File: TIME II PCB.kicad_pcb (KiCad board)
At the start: 2 copper layers, 98 x 98 mm, 91 parts, among them J1 USB_C_Receptacle, J2 SD_Card, J21 Conn_01x02_Male, J3 Conn_01x02_Male, J4 Conn_01x05_Pin, J5 Conn_01x05_Pin, J6 Conn_01x05_Pin, J7 Conn_01x05_Pin, J8 Conn_01x05_Pin, Q1 VNP10N07, Q2 VNP10N07, Q3 VNP10N07, Q4 VNP10N07, Q5 VNP10N07, Q6 NMOS, Q7 PMOS, SW1 PTS647SM38SMTR2LFS, SW2 PTS647SM38SMTR2LFS, U1 ESP32-S2-SOLO, U2 ADP2303, U3 LTC4420CMSE-PBF

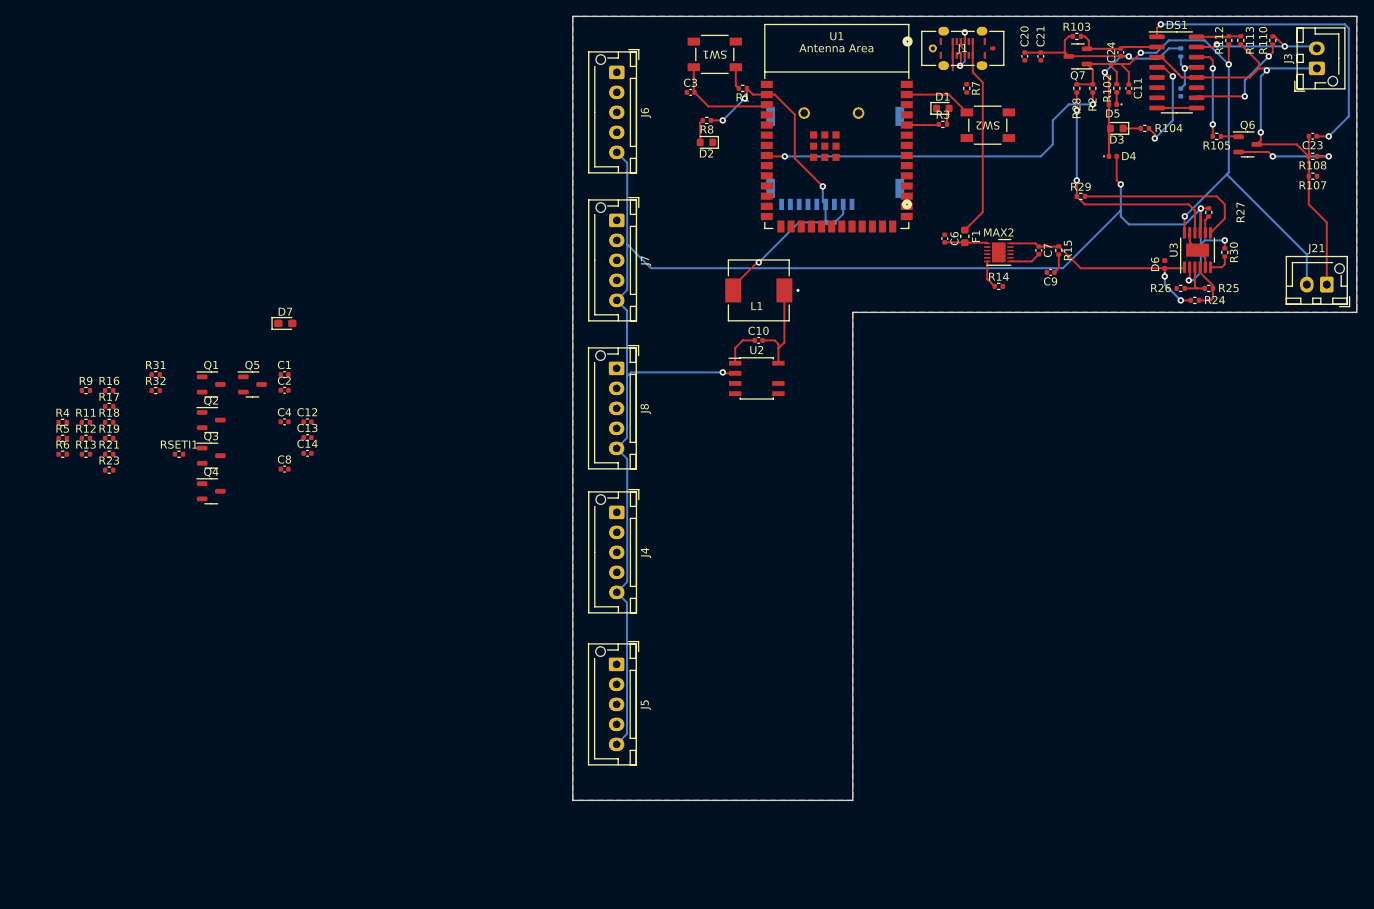
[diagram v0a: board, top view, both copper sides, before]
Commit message: motor driver
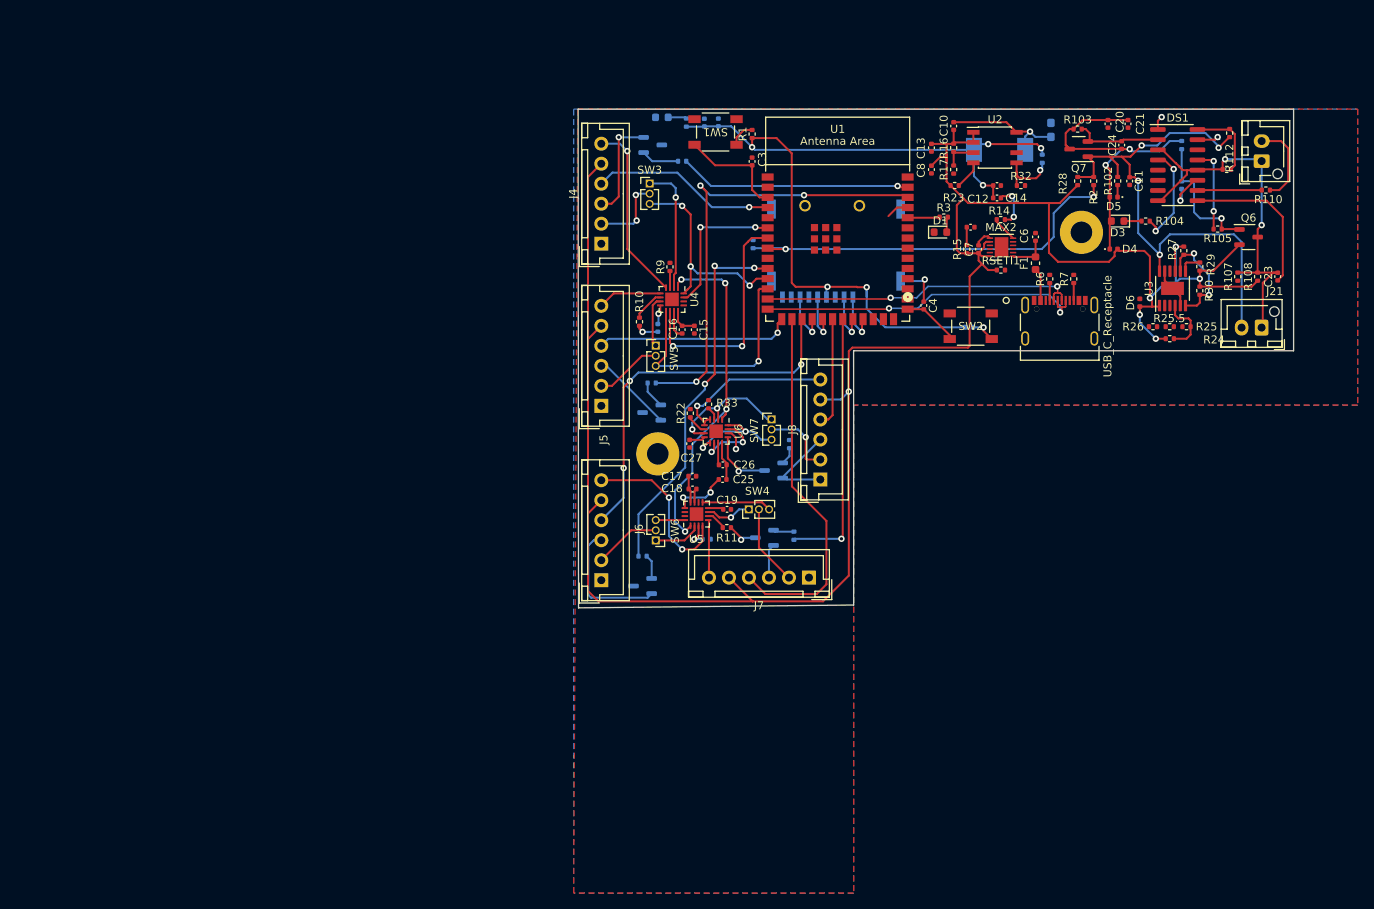
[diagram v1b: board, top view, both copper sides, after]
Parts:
- added ?: , , F.Cu at (150.6, 106.7)
- added C15: 10uF, Capacitor_SMD:C_0402_1005Metric, F.Cu at (155.2, 91.2)
- added C16: 0.01uF, Capacitor_SMD:C_0402_1005Metric, F.Cu at (153.7, 91.2)
- added C17: 10uF, Capacitor_SMD:C_0402_1005Metric, F.Cu at (154.9, 109.5)
- added C18: 0.01uF, Capacitor_SMD:C_0402_1005Metric, F.Cu at (155.0, 111.1)
- added C19: 2.2pF, Capacitor_SMD:C_0402_1005Metric, F.Cu at (159.3, 113.6)
- added C25: 10uF, Capacitor_SMD:C_0402_1005Metric, F.Cu at (158.7, 109.9)
- added C26: 0.01uF, Capacitor_SMD:C_0402_1005Metric, F.Cu at (158.8, 108.1)
- added C27: 2.2pF, Capacitor_SMD:C_0402_1005Metric, F.Cu at (154.6, 105.4)
- added C5: 2.2pF, Capacitor_SMD:C_0402_1005Metric, B.Cu at (150.6, 90.9)
- added R20: 10k, Resistor_SMD:R_0402_1005Metric, B.Cu at (189.5, 90.9)
- added R22: .33, Resistor_SMD:R_0402_1005Metric, F.Cu at (154.7, 101.6)
- added R25.5: 2k, Resistor_SMD:R_0402_1005Metric, F.Cu at (214.6, 90.8)
- added R33: .33, Resistor_SMD:R_0402_1005Metric, F.Cu at (157.0, 100.5)
- added REF**: MountingHole_2.7mm_M2.5_Pad, MountingHole:MountingHole_2.7mm_M2.5_Pad, F.Cu at (203.6, 79.0)
- added SW3: SW_SPDT, Connector_PinHeader_1.27mm:PinHeader_1x03_P1.27mm_Vertical, F.Cu at (149.6, 72.9)
- added SW4: SW_SPDT, Connector_PinHeader_1.27mm:PinHeader_1x03_P1.27mm_Vertical, F.Cu at (162.0, 113.6)
- added SW5: SW_SPDT, Connector_PinHeader_1.27mm:PinHeader_1x03_P1.27mm_Vertical, F.Cu at (150.4, 93.2)
- added SW6: SW_SPDT, Connector_PinHeader_1.27mm:PinHeader_1x03_P1.27mm_Vertical, F.Cu at (150.4, 117.5)
- added SW7: SW_SPDT, Connector_PinHeader_1.27mm:PinHeader_1x03_P1.27mm_Vertical, F.Cu at (164.8, 102.4)
- added U4: ~, Package_DFN_QFN:QFN-16-1EP_3x3mm_P0.5mm_EP1.7x1.7mm, F.Cu at (152.4, 87.4)
- added U5: ~, Package_DFN_QFN:QFN-16-1EP_3x3mm_P0.5mm_EP1.7x1.7mm, F.Cu at (155.5, 114.2)
- added U6: ~, Package_DFN_QFN:QFN-16-1EP_3x3mm_P0.5mm_EP1.7x1.7mm, F.Cu at (157.9, 103.9)
- C1, C2, D2, D7, L1, Q1, Q2, Q3, Q4, Q5, R13, R18, R19, R21, R31, R4, R5, R8: moved to B.Cu
- J1: footprint usb:USB4120-03-C_GCT -> usb:USB4105-GF-A
- J4, J5, J6, J7, J8: value Conn_01x05_Pin -> Conn_01x06_Pin; footprint Connector_JST:JST_XH_B5B-XH-AM_1x05_P2.50mm_Vertical -> Connectors_JST:JST_XH_B06B-XH-A_06x2.50mm_Straight
- R10: value 10k -> .33; moved to F.Cu
- R11, R9: value 10k -> .33
- R12: value 10k -> .33; moved to B.Cu
- R25: value 156k -> 154k
- moved R6 125.3 mm to (199.6, 84.8), turned to 90 degrees
- moved R31 114.0 mm to (198.7, 69.8), turned to -90 degrees
- moved R23 111.5 mm to (187.7, 73.1)
- moved R32 111.1 mm to (196.0, 73.1)
- moved R16 109.8 mm to (187.6, 68.4), turned to -90 degrees
- moved R17 109.6 mm to (187.6, 71.1), turned to -90 degrees
- moved RSETI1 105.3 mm to (193.5, 83.7)
- moved D7 98.7 mm to (199.8, 66.2), turned to 90 degrees
- moved C14 91.9 mm to (193.0, 74.7)
- moved C12 91.1 mm to (193.0, 73.1)
- moved R4 89.1 mm to (162.5, 80.5), turned to 90 degrees
- moved C8 89.1 mm to (184.8, 71.1), turned to -90 degrees
- moved R13 88.0 mm to (167.1, 105.5), turned to 90 degrees
- moved R18 86.8 mm to (167.6, 116.9), turned to -90 degrees
- moved C13 86.0 mm to (184.8, 68.4), turned to -90 degrees
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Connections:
- C10 pad 1: Net-(U2-BST) -> 5v
- C22 pad 1: Net-(DS1-Vdd) -> Net-(Q6-D)
- C23 pad 1: Net-(DS1-Cbias) -> Net-(DS1-Mode)
- C4 pad 1: Net-(U1-GPIO0) -> GND
- C4 pad 2: GND -> Net-(U1-GPIO0)
- C7 pad 1: OR Gate -> 5v
- D6 pad 1: OR Gate -> 5v
- DS1 pad 1: Net-(DS1-Cbias) -> unconnected-(DS1-Cbias-Pad1)
- DS1 pad 14: Net-(DS1-Rt) -> unconnected-(DS1-Rt-Pad14)
- DS1 pad 15: Net-(DS1-THM) -> unconnected-(DS1-THM-Pad15)
- DS1 pad 9: Net-(DS1-CTG) -> Net-(DS1-Mode)
- J2 pad 2: MOSI -> MISO
- J2 pad 7: MISO -> MOSI
- J3 pad 2: Net-(DS1-THM) -> Net-(J3-Pin_2)
- J4 pad 2: SERVO_1 -> ACTUATOR_1
- J5 pad 2: SERVO_2 -> ACTUATOR_2
- J6 pad 2: SERVO_5 -> ACTUATOR_3
- J6 pad 4: therm_5 -> therm_3
- J7 pad 2: SERVO_4 -> ACTUATOR_4
- J8 pad 2: SERVO_3 -> ACTUATOR_5
- J8 pad 4: therm_3 -> therm_5
- MAX2 pad 12: OR Gate -> 5v
- MAX2 pad 8: Net-(MAX2-SETI) -> 5v
- Q2 pad 2: Net-(J6-Pin_3) -> Net-(J8-Pin_3)
- Q5 pad 2: Net-(J8-Pin_3) -> Net-(J6-Pin_3)
- Q6 pad 2: Net-(Q6-G) -> 5v
- R10 pad 1: 3v3 -> Net-(U4-BISEN)
- R10 pad 2: MOSI -> GND
- R101 pad 2: Net-(DS1-Vdd) -> Net-(Q6-D)
- R105 pad 2: Net-(DS1-Rt) -> Net-(DS1-Vdd)
- R108 pad 1: Net-(Q6-G) -> 5v
- R11 pad 1: 3v3 -> Net-(U5-BISEN)
- R11 pad 2: SCK -> GND
- R110 pad 2: Net-(DS1-THM) -> Net-(J3-Pin_2)
- R12 pad 1: 3v3 -> Net-(U5-AISEN)
- R12 pad 2: MISO -> GND
- R15 pad 1: OR Gate -> 5v
- R24 pad 1: OR Gate -> 5v
- R25 pad 2: Net-(U3-CMP1) -> Net-(R25-Pad2)
- R26 pad 1: Net-(U3-CMP1) -> Net-(R25.5-Pad2)
- R27 pad 1: Net-(U3-V2OK) -> Net-(U3-CMPOUT1)
- R28 pad 2: Net-(U3-V2UV) -> 5v
- R29 pad 1: Net-(U3-V2UV) -> 5v
- R5 pad 2: heater_1 -> heater_2
- R9 pad 1: 3v3 -> Net-(U4-AISEN)
- R9 pad 2: SS -> GND
- RSETI1 pad 1: Net-(MAX2-SETI) -> 5v
- SW2 pad 1: unconnected-(SW2-Pad1) -> GND
- SW2 pad 4: heater_1 -> Net-(R20-Pad2)
- U1 pad 10: unconnected-(U1-GPIO17/U1TXD/ADC2_CH6/DAC_1-Pad10) -> heater_3
- U1 pad 11: unconnected-(U1-GPIO18/U1RXD/ADC2_CH7/DAC_2/CLK_OUT3-Pad11) -> SERVO_1
- U1 pad 12: unconnected-(U1-GPIO8/TOUCH8/ADC1_CH7-Pad12) -> SERVO_2
- U1 pad 16: unconnected-(U1-GPIO46-Pad16) -> therm_4
- U1 pad 18: unconnected-(U1-GPIO10/TOUCH10/ADC1_CH9/FSPICS0/FSPIIO4-Pad18) -> MOSI
- U1 pad 19: SERVO_1 -> SCK
- U1 pad 2: 3v3 -> unconnected-(U1-3V3-Pad2)
- U1 pad 20: unconnected-(U1-GPIO12/TOUCH12/ADC2_CH1/FSPICLK/FSPIIO6-Pad20) -> therm_5
- U1 pad 21: SERVO_2 -> heater_4
- U1 pad 22: unconnected-(U1-GPIO14/TOUCH14/ADC2_CH3/FSPIWP/FSPIDQS-Pad22) -> MISO
- U1 pad 23: therm_5 -> SS
- U1 pad 24: unconnected-(U1-SPIIO4/GPIO33/FSPIHD-Pad24) -> SERVO_3A
- U1 pad 25: unconnected-(U1-SPIIO5/GPIO34/FSPICS0-Pad25) -> SERVO_4A
- U1 pad 26: heater_4 -> unconnected-(U1-GPIO45-Pad26)
- U1 pad 28: unconnected-(U1-SPIIO6/GPIO35/FSPID-Pad28) -> SERVO_5A
- U1 pad 34: heater_3 -> unconnected-(U1-MTDI/GPIO41/CLK_OUT1-Pad34)
- U1 pad 35: therm_1 -> unconnected-(U1-MTMS/GPIO42-Pad35)
- U1 pad 38: heater_1 -> heater_2
- U1 pad 4: therm_4 -> therm_1
- U1 pad 6: unconnected-(U1-GPIO6/TOUCH6/ADC1_CH5-Pad6) -> SERVO_1A
- U1 pad 7: unconnected-(U1-GPIO7/TOUCH7/ADC1_CH6-Pad7) -> SERVO_2A
- U1 pad 9: unconnected-(U1-GPIO16/U0CTS/ADC2_CH5/XTAL_32K_N-Pad9) -> MOT_CON
- U2 pad 1: Net-(U2-BST) -> 5v
- U3 pad 1: OR Gate -> 5v
- U3 pad 10: Net-(U3-V2UV) -> 5v
- U3 pad 13: (no net) -> GND
- U3 pad 2: 5v -> unconnected-(U3-V2TEST-Pad2)
- U3 pad 3: Net-(U3-CMP1) -> unconnected-(U3-CMP1-Pad3)
- U3 pad 8: Net-(U3-V2OK) -> Net-(U3-CMPOUT1)
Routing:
- net 5v: track 196.9 -> 275.7 mm, vias 5 -> 6
- net 3v3: track 44.7 -> 106.5 mm, vias 4 -> 6
- net heater_2: track 0.00 -> 57.0 mm, vias 0 -> 3
- net heater_3: track 0.00 -> 47.0 mm, vias 0 -> 3
- net therm_3: track 0.00 -> 46.9 mm, vias 0 -> 3
- net therm_4: track 0.00 -> 46.3 mm
- net MOT_CON: track 0.00 -> 43.7 mm, vias 0 -> 4
- net Net-(DS1-Cbias): track 41.5 -> 0.00 mm, vias 2 -> 0
- net GND: track 9.03 -> 50.0 mm, vias 0 -> 9
- net D+: track 1.94 -> 42.1 mm, vias 0 -> 2
- net heater_4: track 0.00 -> 33.5 mm, vias 0 -> 1
- net D-: track 6.92 -> 40.3 mm
- net Net-(U3-V2UV): track 31.3 -> 0.00 mm, vias 2 -> 0
- net SERVO_2: track 0.00 -> 30.6 mm, vias 0 -> 1
- net OR Gate: track 29.2 -> 0.00 mm, vias 2 -> 0
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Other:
- board size 98 x 98 mm -> 89.4 x 62.3 mm

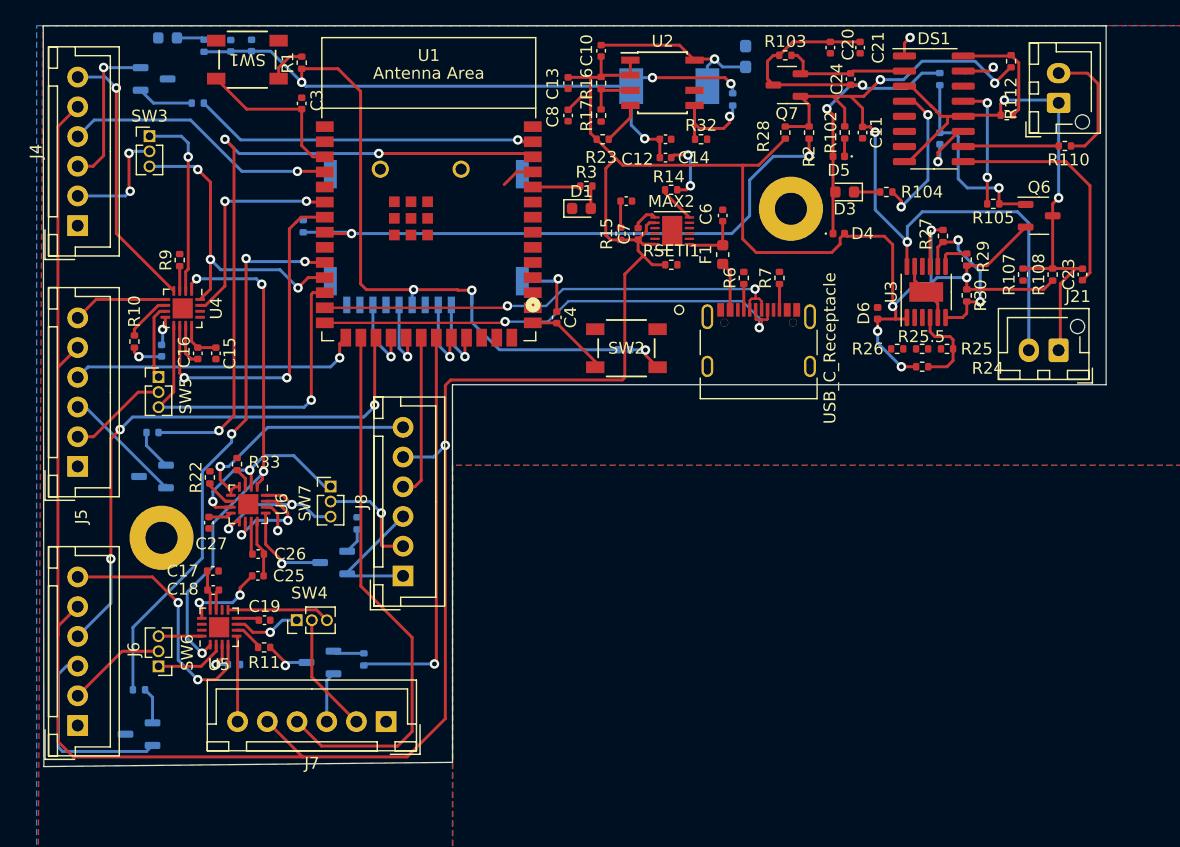
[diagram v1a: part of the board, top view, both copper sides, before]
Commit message: done?
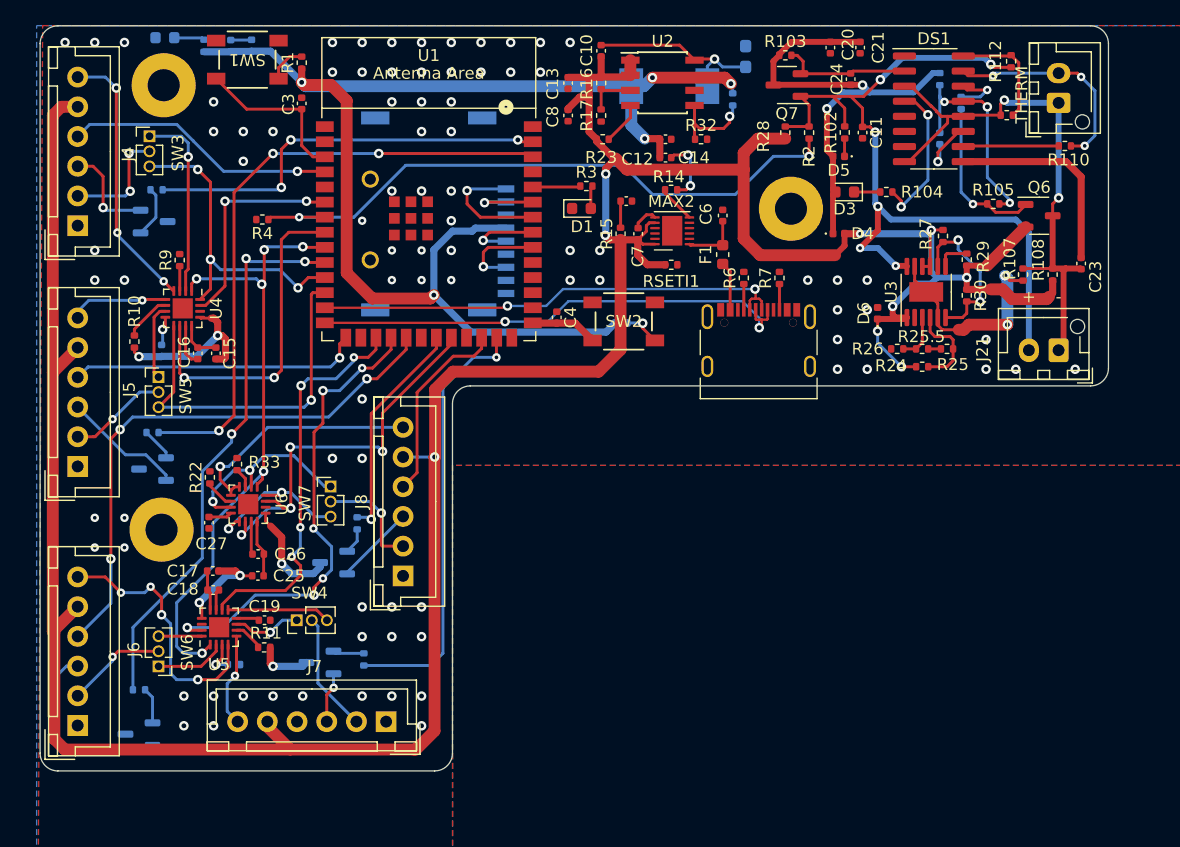
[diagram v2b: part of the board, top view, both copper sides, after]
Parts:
- added ?: , , F.Cu at (150.8, 68.6)
- added R34: 86K, Resistor_SMD:R_0402_1005Metric, B.Cu at (217.9, 70.1)
- R101: value R -> 150
- R102: value R -> 220
- R103, R104: value R -> 470
- R107: value 7 -> .25
- R108, R110: value R -> 10K
- R113: value R -> 100K
- R4: moved to F.Cu
- moved Q4 12.0 mm to (150.0, 80.1)
- moved R21 8.08 mm to (150.2, 77.4)
- moved R4 3.49 mm to (159.1, 79.9), turned to 180 degrees
- moved R20 2.27 mm to (189.3, 88.6)
- moved SW2 2.27 mm to (189.5, 88.5)
- moved J2 1.05 mm to (171.9, 79.4), turned to 90 degrees
- moved C23 0.93 mm to (228.0, 83.6), turned to -90 degrees
- moved ? 0.68 mm to (150.6, 106.0)
- moved Q1 0.62 mm to (149.9, 100.9)
- moved D2 0.23 mm to (150.9, 64.6)
- turned R105 to 0 degrees
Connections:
- ? pad 1: (no net) -> GND
- C22 pad 1: Net-(Q6-D) -> Net-(DS1-Vdd)
- DS1 pad 14: unconnected-(DS1-Rt-Pad14) -> Net-(DS1-Rt)
- DS1 pad 15: unconnected-(DS1-THM-Pad15) -> Net-(DS1-THM)
- J3 pad 2: Net-(J3-Pin_2) -> Net-(DS1-THM)
- R101 pad 2: Net-(Q6-D) -> Net-(DS1-Vdd)
- R110 pad 2: Net-(J3-Pin_2) -> Net-(DS1-THM)
- R25.5 pad 2: Net-(R25.5-Pad2) -> Net-(U3-CMP1)
- R26 pad 1: Net-(R25.5-Pad2) -> Net-(U3-CMP1)
- REF** pad 1: (no net) -> GND
- U1 pad 16: therm_4 -> unconnected-(U1-GPIO46-Pad16)
- U1 pad 17: therm_3 -> SERVO_4A
- U1 pad 18: MOSI -> SERVO_3A
- U1 pad 19: SCK -> therm_3
- U1 pad 20: therm_5 -> unconnected-(U1-GPIO12/TOUCH12/ADC2_CH1/FSPICLK/FSPIIO6-Pad20)
- U1 pad 21: heater_4 -> heater_5
- U1 pad 22: MISO -> SERVO_5A
- U1 pad 23: SS -> unconnected-(U1-GPIO21-Pad23)
- U1 pad 24: SERVO_3A -> therm_5
- U1 pad 25: SERVO_4A -> heater_4
- U1 pad 28: SERVO_5A -> unconnected-(U1-SPIIO6/GPIO35/FSPID-Pad28)
- U1 pad 32: unconnected-(U1-MTCK/GPIO39/CLK_OUT3-Pad32) -> MOSI
- U1 pad 33: unconnected-(U1-MTDO/GPIO40/CLK_OUT2-Pad33) -> SCK
- U1 pad 34: unconnected-(U1-MTDI/GPIO41/CLK_OUT1-Pad34) -> SS
- U1 pad 35: unconnected-(U1-MTMS/GPIO42-Pad35) -> MISO
- U1 pad 37: heater_5 -> unconnected-(U1-U0TXD/GPIO43/CLK_OUT1-Pad37)
- U1 pad 7: SERVO_2A -> V_MON
- U1 pad 8: V_MON -> SERVO_2A
- U3 pad 3: unconnected-(U3-CMP1-Pad3) -> Net-(U3-CMP1)
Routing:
- net therm_4: track 46.3 -> 0.00 mm
- net SERVO_3A: track 0.00 -> 40.1 mm, vias 0 -> 6
- net SERVO_4A: track 0.00 -> 33.4 mm, vias 0 -> 4
- net SERVO_5A: track 8.55 -> 33.2 mm, vias 2 -> 4
- net GND: track 50.0 -> 70.4 mm, vias 9 -> 95
- net Net-(DS1-THM): track 0.00 -> 18.1 mm, vias 0 -> 3
- net heater_5: track 2.85 -> 18.8 mm, vias 0 -> 1
- net Net-(J3-Pin_2): track 10.9 -> 0.00 mm
- net MOT_CON: track 43.7 -> 53.3 mm, vias 4 -> 6
- net Net-(DS1-Vdd): track 10.6 -> 18.2 mm, vias 2 -> 3
- net heater_1: track 29.0 -> 34.8 mm, vias 1 -> 3
- net heater_2: track 57.0 -> 51.9 mm
- net Net-(J4-Pin_3): track 13.1 -> 8.37 mm
- net 5v: track 275.7 -> 280.4 mm, vias 6 -> 9
- net Net-(DS1-Rt): track 0.00 -> 4.59 mm, vias 0 -> 1
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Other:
- board size 89.4 x 62.3 mm -> 89.9 x 62.7 mm
- board text added: "+"
- board text added: "-"
- board text added: "THERM"
